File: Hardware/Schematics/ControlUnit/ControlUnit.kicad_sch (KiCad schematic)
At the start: 9 parts

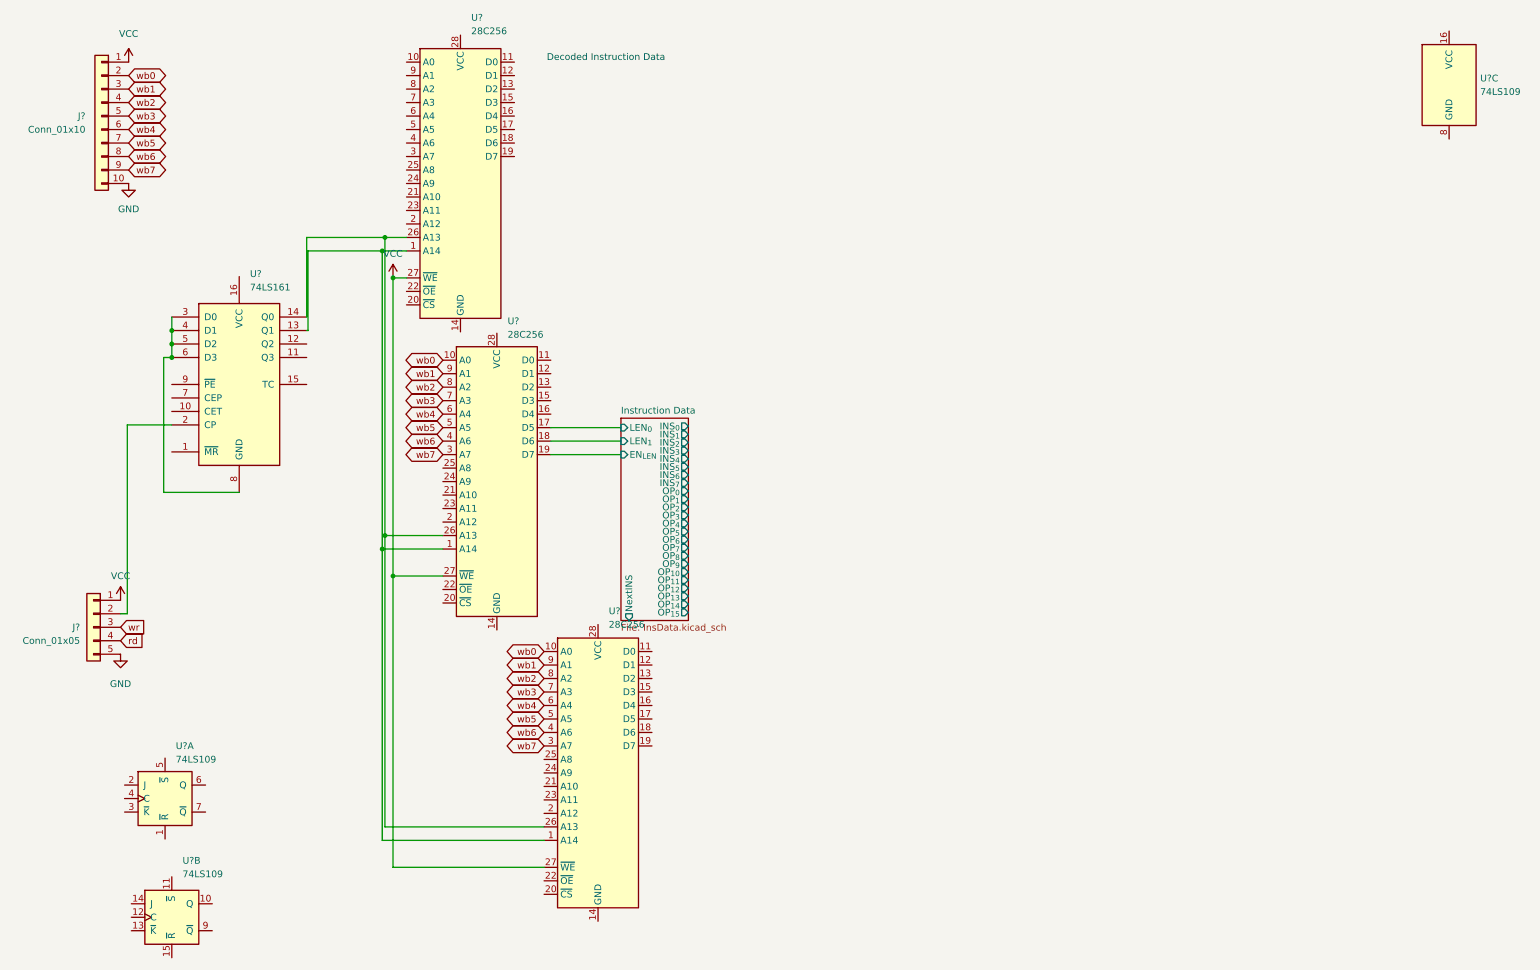
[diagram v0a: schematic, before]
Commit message: Interim
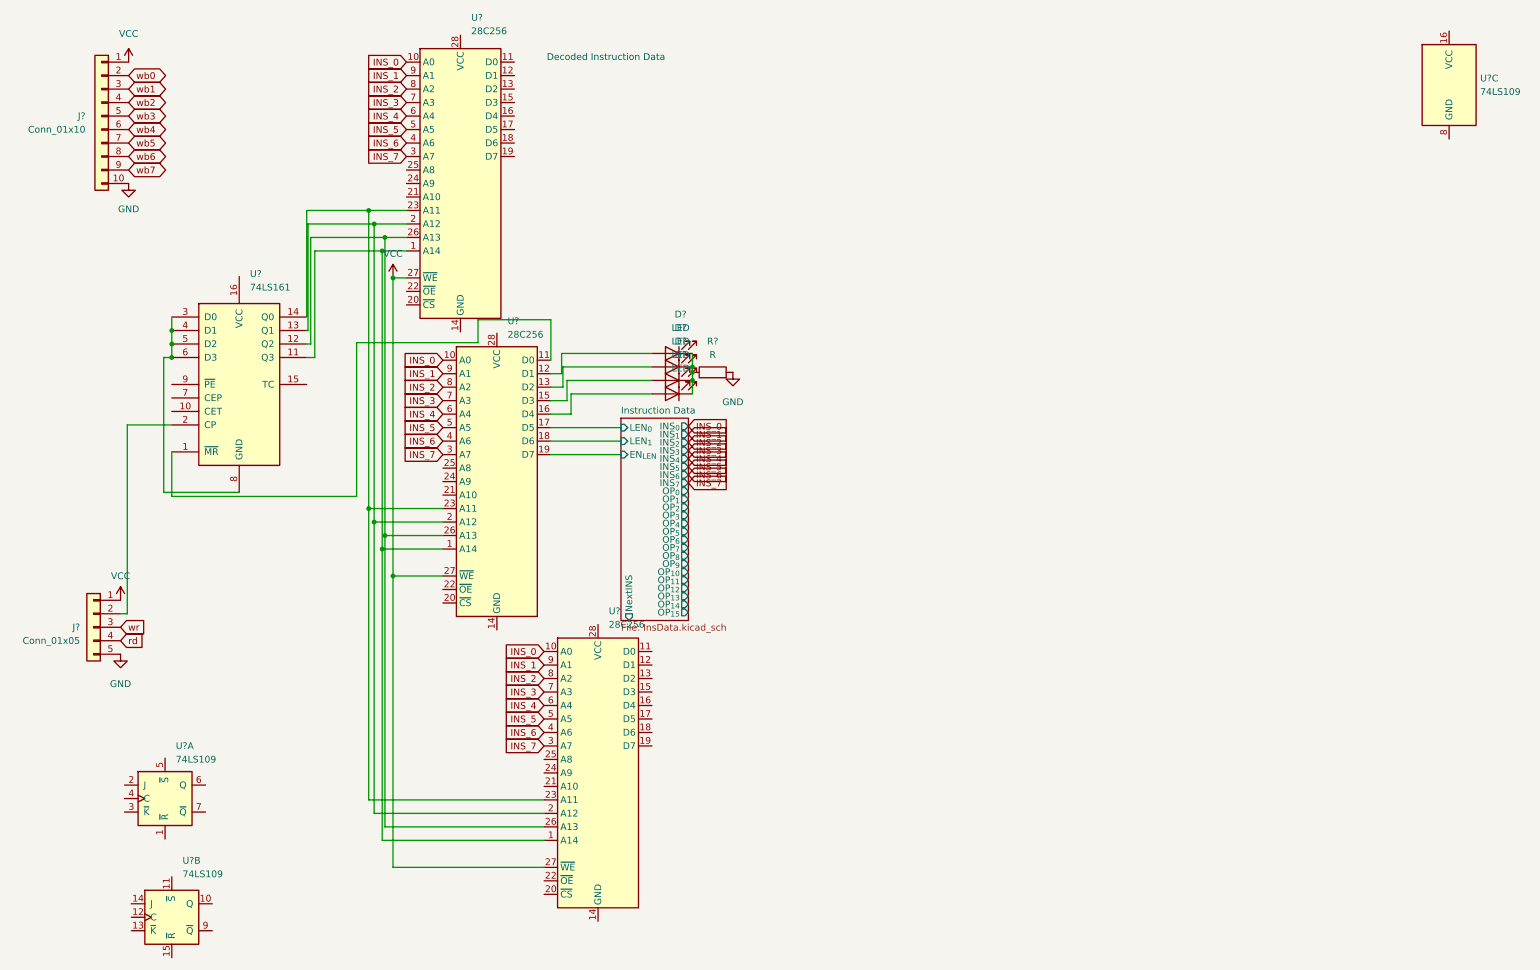
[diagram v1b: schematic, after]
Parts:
- added D? (x4): LED, LED_THT:LED_D3.0mm, symbol Device:LED
- added R?: R, symbol Device:R
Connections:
- net GND: now also R?.2
- net wb0: no longer U?.10 (A0), U?.10 (A0)
- net wb1: no longer U?.9 (A1), U?.9 (A1)
- net wb2: no longer U?.8 (A2), U?.8 (A2)
- net wb3: no longer U?.7 (A3), U?.7 (A3)
- net wb4: no longer U?.6 (A4), U?.6 (A4)
- net wb5: no longer U?.5 (A5), U?.5 (A5)
- net wb6: no longer U?.4 (A6), U?.4 (A6)
- net wb7: no longer U?.3 (A7), U?.3 (A7)
- net at U?.1 (~{MR}): now also U?.11 (D0)
- net at U?.11 (Q3): now also U?.1 (A14), U?.1 (A14), U?.1 (A14)
- net at U?.12 (Q2): now also U?.26 (A13), U?.26 (A13), U?.26 (A13)
- net INS_0: now reaches U?.10 (A0)
- net INS_0: now also U?.10 (A0), U?.10 (A0)
- net at U?.2 (A12): now also U?.13 (Q1), U?.2 (A12), U?.2 (A12)
- net at U?.23 (A11): now also U?.14 (Q0), U?.23 (A11), U?.23 (A11)
- net INS_7: now reaches U?.3 (A7)
- net INS_7: now also U?.3 (A7), U?.3 (A7)
- net INS_6: now reaches U?.4 (A6)
- net INS_6: now also U?.4 (A6), U?.4 (A6)
- net INS_5: now reaches U?.5 (A5)
- net INS_5: now also U?.5 (A5), U?.5 (A5)
- net INS_4: now reaches U?.6 (A4)
- net INS_4: now also U?.6 (A4), U?.6 (A4)
- net INS_3: now reaches U?.7 (A3)
- net INS_3: now also U?.7 (A3), U?.7 (A3)
- net INS_2: now reaches U?.8 (A2)
- net INS_2: now also U?.8 (A2), U?.8 (A2)
- net INS_1: now reaches U?.9 (A1)
- net INS_1: now also U?.9 (A1), U?.9 (A1)
- net at U?.12 (D1): now also D?.2 (A)
- net at U?.13 (D2): now also D?.2 (A)
- net at U?.15 (D3): now also D?.2 (A)
- net at U?.16 (D4): now also D?.2 (A)
- new net: D?.1 (K), D?.1 (K), D?.1 (K), D?.1 (K), R?.1
